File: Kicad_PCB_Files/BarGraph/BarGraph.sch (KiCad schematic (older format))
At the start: 11 parts, among them U1 LED-Bar-Graph

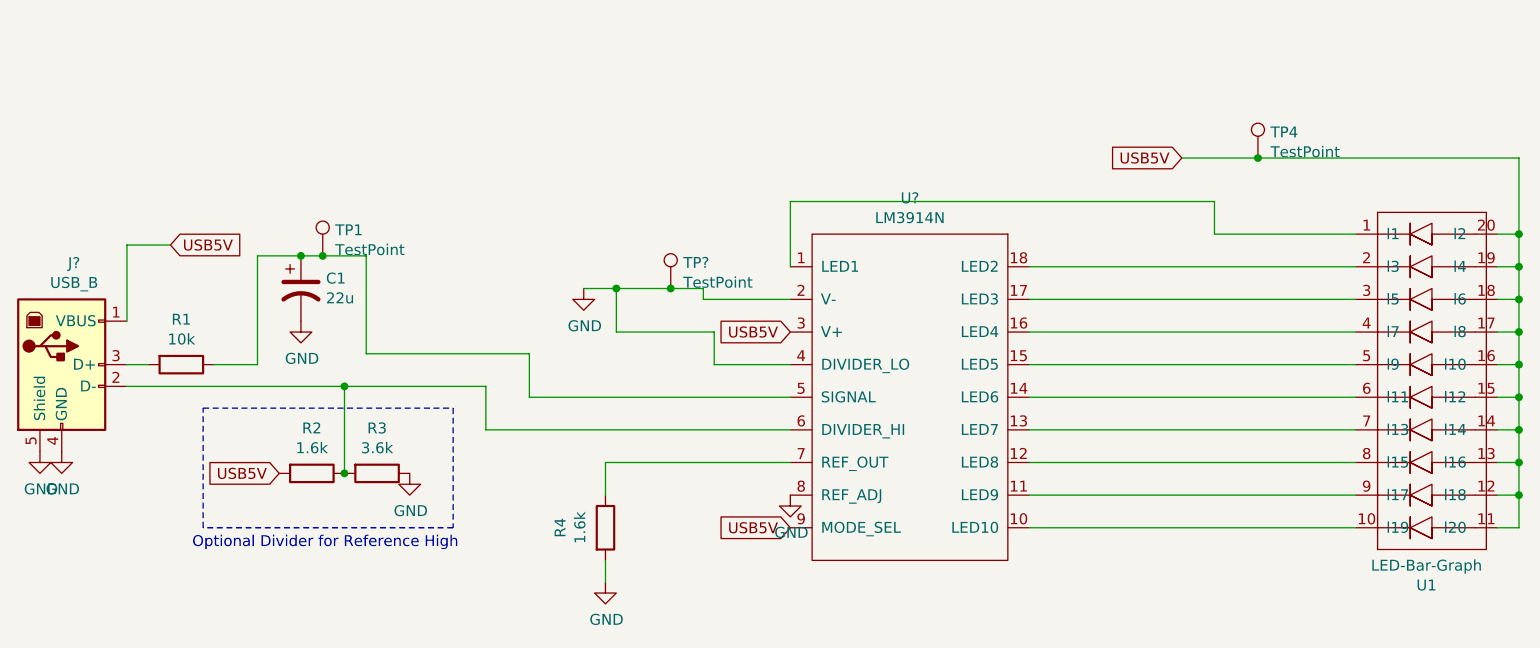
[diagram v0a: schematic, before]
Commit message: Add files via upload
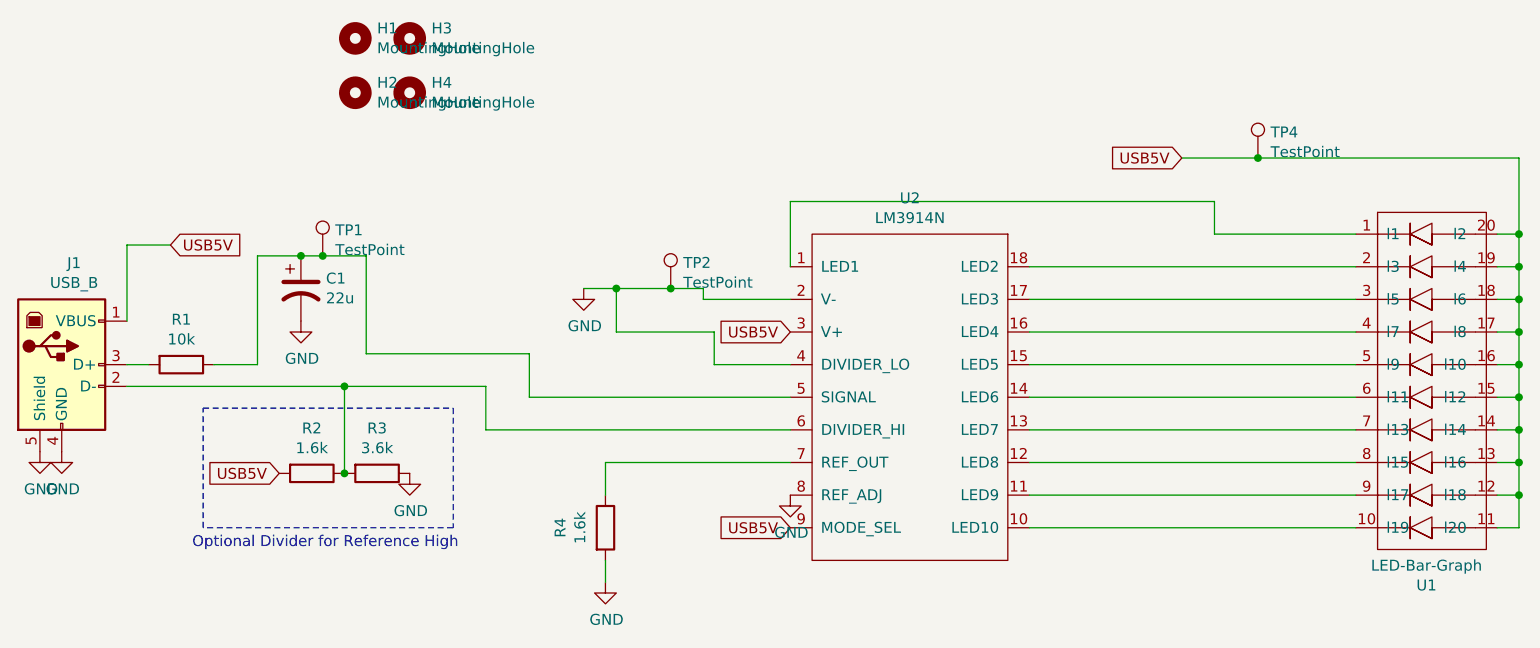
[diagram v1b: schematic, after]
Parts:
- added H1, H2, H3, H4: MountingHole, MountingHole:MountingHole_4mm_Pad, symbol Mechanical:MountingHole
- R1: footprint Resistor_THT:R_Axial_DIN0309_L9.0mm_D3.2mm_P12.70mm_Horizontal -> Resistor_THT:R_Axial_DIN0207_L6.3mm_D2.5mm_P10.16mm_Horizontal
- gave numbers to parts that had none: 3
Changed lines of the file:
@@
 F 0 "R1" V 2943 3950 50  0000 C CNN
 F 1 "10k" V 3034 3950 50  0000 C CNN
-F 2 "Resistor_THT:R_Axial_DIN0309_L9.0mm_D3.2mm_P12.70mm_Horizontal" V 3080 3950 50  0001 C CNN
+F 2 "Resistor_THT:R_Axial_DIN0207_L6.3mm_D2.5mm_P10.16mm_Horizontal" V 3080 3950 50  0001 C CNN
 F 3 "~" H 3150 3950 50  0001 C CNN
 	1    3150 3950
@@
 Optional Divider for Reference High
 $Comp
-L lm3914n:LM3914N U?
+L lm3914n:LM3914N U2
 U 1 1 5D46F6ED
 P 6500 4100
-F 0 "U?" H 6500 5015 50  0000 C CNN
+F 0 "U2" H 6500 5015 50  0000 C CNN
 F 1 "LM3914N" H 6500 4924 50  0000 C CNN
 F 2 "Package_DIP:DIP-18_W7.62mm_Socket_LongPads" H 6500 3900 50  0001 C CNN
@@
 	5950 3200 5950 3500
 $Comp
-L Connector:USB_B J?
+L Connector:USB_B J1
 U 1 1 5D489EC6
 P 2600 3950
-F 0 "J?" H 2657 4417 50  0000 C CNN
+F 0 "J1" H 2657 4417 50  0000 C CNN
 F 1 "USB_B" H 2657 4326 50  0000 C CNN
 F 2 "SmartGluttonV1:USB_B_Molex_USB-67068-xx1x_StraightTab_Horizontal" H 2750 3900 50  0001 C CNN
@@
 Wire Wire Line
 	7050 3500 8550 3500
-Text GLabel 5950 4700 0    50   Input ~ 0
-USB5V
-$Comp
-L Connector:TestPoint TP?
+$Comp
+L Connector:TestPoint TP2
 U 1 1 5D467D46
 P 5400 3600
-F 0 "TP?" H 5458 3718 50  0000 L CNN
+F 0 "TP2" H 5458 3718 50  0000 L CNN
 F 1 "TestPoint" H 5458 3627 50  0000 L CNN
 F 2 "TestPoint:TestPoint_Pad_2.5x2.5mm" H 5600 3600 50  0001 C CNN
@@
 Wire Wire Line
 	5400 3600 5550 3600
+Text GLabel 5950 4700 0    50   Input ~ 0
+USB5V
+$Comp
+L Mechanical:MountingHole H1
+U 1 1 5D46FB90
+P 3950 2450
+F 0 "H1" H 4050 2496 50  0000 L CNN
+F 1 "MountingHole" H 4050 2405 50  0000 L CNN
+F 2 "MountingHole:MountingHole_4mm_Pad" H 3950 2450 50  0001 C CNN
+F 3 "~" H 3950 2450 50  0001 C CNN
+	1    3950 2450
+	1    0    0    -1
+$EndComp
+$Comp
+L Mechanical:MountingHole H3
+U 1 1 5D4716A5
+P 4200 2450
+F 0 "H3" H 4300 2496 50  0000 L CNN
+F 1 "MountingHole" H 4300 2405 50  0000 L CNN
+F 2 "MountingHole:MountingHole_4mm_Pad" H 4200 2450 50  0001 C CNN
+F 3 "~" H 4200 2450 50  0001 C CNN
+	1    4200 2450
+	1    0    0    -1
+$EndComp
+$Comp
+L Mechanical:MountingHole H2
+U 1 1 5D4718D9
+P 3950 2700
+F 0 "H2" H 4050 2746 50  0000 L CNN
+F 1 "MountingHole" H 4050 2655 50  0000 L CNN
+F 2 "MountingHole:MountingHole_4mm_Pad" H 3950 2700 50  0001 C CNN
+F 3 "~" H 3950 2700 50  0001 C CNN
+	1    3950 2700
+	1    0    0    -1
+$EndComp
+$Comp
+L Mechanical:MountingHole H4
+U 1 1 5D471C37
+P 4200 2700
+F 0 "H4" H 4300 2746 50  0000 L CNN
+F 1 "MountingHole" H 4300 2655 50  0000 L CNN
+F 2 "MountingHole:MountingHole_4mm_Pad" H 4200 2700 50  0001 C CNN
+F 3 "~" H 4200 2700 50  0001 C CNN
+	1    4200 2700
+	1    0    0    -1
+$EndComp
 $EndSCHEMATC

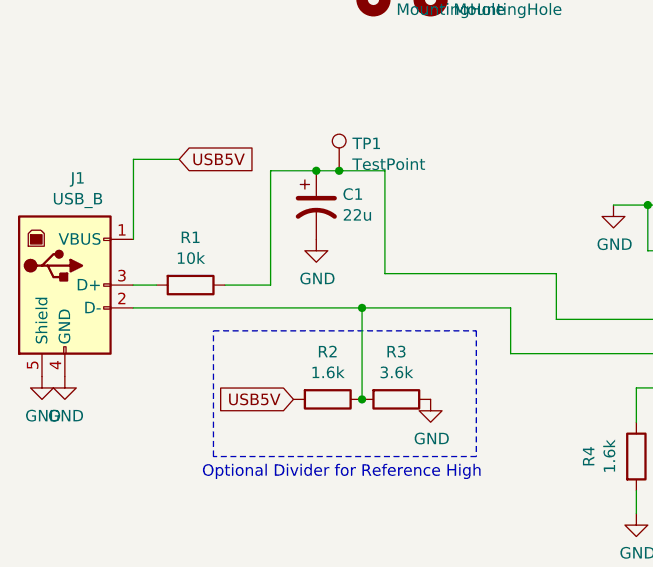
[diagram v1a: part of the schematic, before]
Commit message: Add files via upload
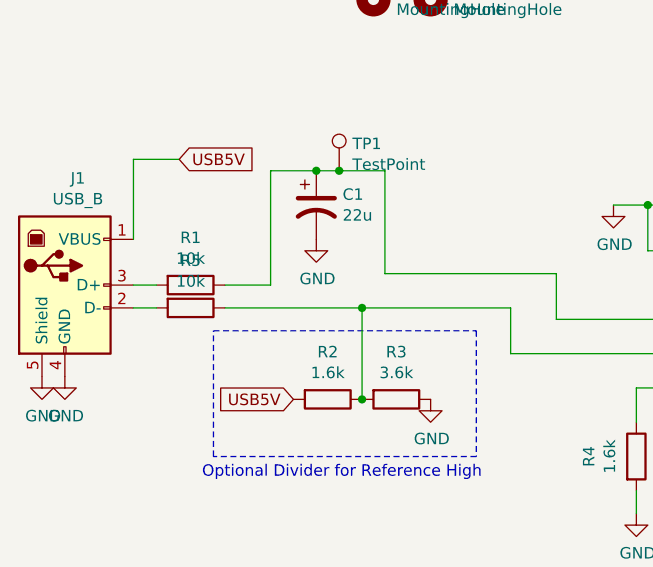
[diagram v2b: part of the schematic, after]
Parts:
- added R5: 10k, Resistor_THT:R_Axial_DIN0207_L6.3mm_D2.5mm_P10.16mm_Horizontal, symbol Device:R
- H1, H2, H3, H4: footprint MountingHole:MountingHole_4mm_Pad -> MountingHole:MountingHole_4mm
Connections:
- net at R2.1, R3.2, U2.6 (DIVIDER_HI): now also R5.1; no longer J1.2 (D-)
- new net: J1.2 (D-), R5.2
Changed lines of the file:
@@
 	1    0    0    -1
 $EndComp
-Wire Wire Line
-	2900 4050 3900 4050
 Connection ~ 3900 4450
 Wire Wire Line
@@
 Wire Wire Line
 	4550 4250 5950 4250
-Connection ~ 3900 4050
 Wire Wire Line
 	4000 3900 4750 3900
@@
 F 0 "H1" H 4050 2496 50  0000 L CNN
 F 1 "MountingHole" H 4050 2405 50  0000 L CNN
-F 2 "MountingHole:MountingHole_4mm_Pad" H 3950 2450 50  0001 C CNN
+F 2 "MountingHole:MountingHole_4mm" H 3950 2450 50  0001 C CNN
 F 3 "~" H 3950 2450 50  0001 C CNN
 	1    3950 2450
@@
 F 0 "H3" H 4300 2496 50  0000 L CNN
 F 1 "MountingHole" H 4300 2405 50  0000 L CNN
-F 2 "MountingHole:MountingHole_4mm_Pad" H 4200 2450 50  0001 C CNN
+F 2 "MountingHole:MountingHole_4mm" H 4200 2450 50  0001 C CNN
 F 3 "~" H 4200 2450 50  0001 C CNN
 	1    4200 2450
@@
 F 0 "H2" H 4050 2746 50  0000 L CNN
 F 1 "MountingHole" H 4050 2655 50  0000 L CNN
-F 2 "MountingHole:MountingHole_4mm_Pad" H 3950 2700 50  0001 C CNN
+F 2 "MountingHole:MountingHole_4mm" H 3950 2700 50  0001 C CNN
 F 3 "~" H 3950 2700 50  0001 C CNN
 	1    3950 2700
@@
 F 0 "H4" H 4300 2746 50  0000 L CNN
 F 1 "MountingHole" H 4300 2655 50  0000 L CNN
-F 2 "MountingHole:MountingHole_4mm_Pad" H 4200 2700 50  0001 C CNN
+F 2 "MountingHole:MountingHole_4mm" H 4200 2700 50  0001 C CNN
 F 3 "~" H 4200 2700 50  0001 C CNN
 	1    4200 2700
 	1    0    0    -1
 $EndComp
+$Comp
+L Device:R R5
+U 1 1 5D623D89
+P 3150 4050
+F 0 "R5" V 2943 4050 50  0000 C CNN
+F 1 "10k" V 3034 4050 50  0000 C CNN
+F 2 "Resistor_THT:R_Axial_DIN0207_L6.3mm_D2.5mm_P10.16mm_Horizontal" V 3080 4050 50  0001 C CNN
+F 3 "~" H 3150 4050 50  0001 C CNN
+	1    3150 4050
+	0    1    1    0
+$EndComp
+Wire Wire Line
+	2900 4050 3000 4050
+Wire Wire Line
+	3300 4050 3900 4050
+Connection ~ 3900 4050
 $EndSCHEMATC
